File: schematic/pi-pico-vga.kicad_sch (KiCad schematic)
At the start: 33 parts, among them J1 VGA, J2 USB Keyboard, J3 Micro_SD_Card, J4 Power, J5 UART, J6 External, J7 Jack-DC, SW1 Power switch, SW2 User, SW3 Microswitch, U1 DS1307+, U2 Level Shift, Y1 32.768 Hz

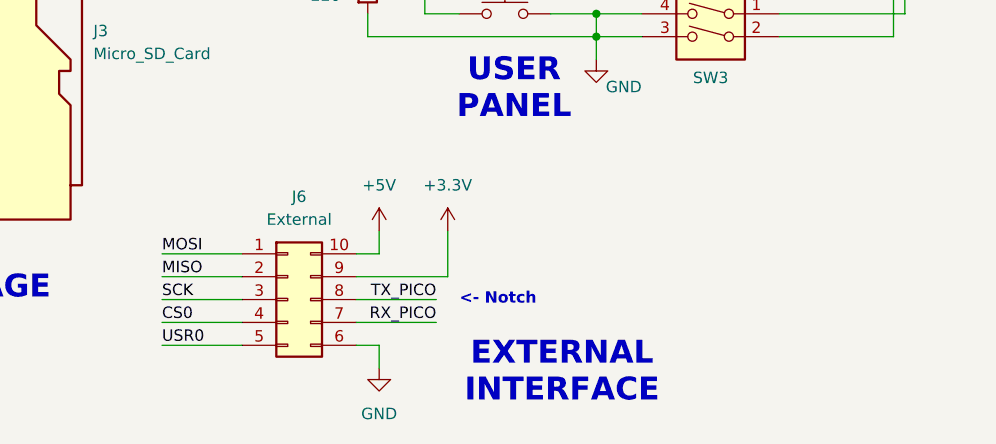
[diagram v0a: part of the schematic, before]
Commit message: .
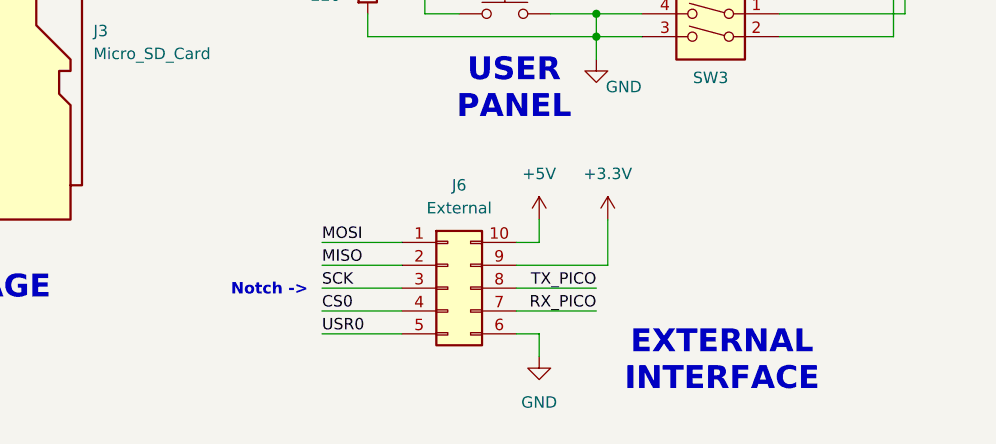
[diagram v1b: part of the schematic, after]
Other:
- note added: "Notch ->"
- note removed: "<- Notch"
- moved on the sheet: J6
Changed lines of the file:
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@@
 	(text "EXTERNAL\nINTERFACE"
 		(exclude_from_sim no)
-		(at 115.57 191.008 0)
+		(at 133.35 189.738 0)
 		(effects
 			(font
@@
 		)
 	)
-	(text "<- Notch"
+	(text "USER\nPANEL"
 		(exclude_from_sim no)
-		(at 108.458 182.88 0)
+		(at 110.236 159.512 0)
 		(effects
 			(font
-				(size 1.27 1.27)
-				(thickness 0.254)
+				(size 2.54 2.54)
+				(thickness 0.508)
 				(bold yes)
 			)
 		)
 	)
-	(text "USER\nPANEL"
+	(text "Notch ->"
 		(exclude_from_sim no)
-		(at 110.236 159.512 0)
+		(at 83.058 181.864 0)
 		(effects
 			(font
-				(size 2.54 2.54)
-				(thickness 0.508)
+				(size 1.27 1.27)
+				(thickness 0.254)
 				(bold yes)
 			)
@@
 	(wire
 		(pts
-			(xy 102.87 175.26) (xy 102.87 180.34)
+			(xy 120.65 173.99) (xy 120.65 179.07)
 		)
 		(stroke
@@
 	(wire
 		(pts
-			(xy 102.87 180.34) (xy 92.71 180.34)
+			(xy 120.65 179.07) (xy 110.49 179.07)
 		)
 		(stroke
@@
 	(wire
 		(pts
-			(xy 95.25 177.8) (xy 92.71 177.8)
+			(xy 113.03 176.53) (xy 110.49 176.53)
 		)
 		(stroke
@@
 	(wire
 		(pts
-			(xy 71.12 180.34) (xy 80.01 180.34)
+			(xy 88.9 179.07) (xy 97.79 179.07)
 		)
 		(stroke
@@
 	(wire
 		(pts
-			(xy 71.12 177.8) (xy 80.01 177.8)
+			(xy 88.9 176.53) (xy 97.79 176.53)
 		)
 		(stroke
@@
 	(wire
 		(pts
-			(xy 95.25 190.5) (xy 95.25 187.96)
+			(xy 113.03 189.23) (xy 113.03 186.69)
 		)
 		(stroke
@@
 	(wire
 		(pts
-			(xy 71.12 182.88) (xy 80.01 182.88)
+			(xy 88.9 181.61) (xy 97.79 181.61)
 		)
 		(stroke
@@
 	(wire
 		(pts
-			(xy 95.25 175.26) (xy 95.25 177.8)
+			(xy 113.03 173.99) (xy 113.03 176.53)
 		)
 		(stroke
@@
 	(wire
 		(pts
-			(xy 95.25 187.96) (xy 92.71 187.96)
+			(xy 113.03 186.69) (xy 110.49 186.69)
 		)
 		(stroke
@@
 	(wire
 		(pts
-			(xy 101.6 182.88) (xy 92.71 182.88)
+			(xy 119.38 181.61) (xy 110.49 181.61)
 		)
 		(stroke
@@
 	(wire
 		(pts
-			(xy 71.12 187.96) (xy 80.01 187.96)
+			(xy 88.9 186.69) (xy 97.79 186.69)
 		)
 		(stroke
@@
 	(wire
 		(pts
-			(xy 71.12 185.42) (xy 80.01 185.42)
+			(xy 88.9 184.15) (xy 97.79 184.15)
 		)
 		(stroke
@@
 	(wire
 		(pts
-			(xy 101.6 185.42) (xy 92.71 185.42)
+			(xy 119.38 184.15) (xy 110.49 184.15)
 		)
 		(stroke
@@
 	)
 	(label "RX_PICO"
-		(at 101.6 185.42 180)
+		(at 119.38 184.15 180)
 		(effects
 			(font
@@
 	)
 	(label "MISO"
-		(at 71.12 180.34 0)
+		(at 88.9 179.07 0)
 		(effects
 			(font
@@
 	)
 	(label "USR0"
-		(at 71.12 187.96 0)
+		(at 88.9 186.69 0)
 		(effects
 			(font
@@
 	)
 	(label "SCK"
-		(at 71.12 182.88 0)
+		(at 88.9 181.61 0)
 		(effects
 			(font
@@
 	)
 	(label "TX_PICO"
-		(at 101.6 182.88 180)
+		(at 119.38 181.61 180)
 		(effects
 			(font
@@
 	)
 	(label "CS0"
-		(at 71.12 185.42 0)
+		(at 88.9 184.15 0)
 		(effects
 			(font
@@
 	)
 	(label "MOSI"
-		(at 71.12 177.8 0)
+		(at 88.9 176.53 0)
 		(effects
 			(font
@@
 	(symbol
 		(lib_id "power:+3.3V")
-		(at 102.87 175.26 0)
+		(at 120.65 173.99 0)
 		(unit 1)
 		(exclude_from_sim no)
@@
 		(fields_autoplaced yes)
 		(property "Reference" "#PWR021"
-			(at 102.87 179.07 0)
+			(at 120.65 177.8 0)
 			(effects
 				(font
@@
 		)
 		(property "Value" "+3.3V"
-			(at 102.87 170.18 0)
+			(at 120.65 168.91 0)
 			(effects
 				(font
@@
 		)
 		(property "Footprint" ""
-			(at 102.87 175.26 0)
+			(at 120.65 173.99 0)
 			(effects
 				(font
@@
 		)
 		(property "Datasheet" ""
-			(at 102.87 175.26 0)
+			(at 120.65 173.99 0)
 			(effects
 				(font
@@
 		)
 		(property "Description" "Power symbol creates a global label with name \"+3.3V\""
-			(at 102.87 175.26 0)
+			(at 120.65 173.99 0)
 			(effects
 				(font
@@
 	(symbol
 		(lib_id "power:GND")
-		(at 95.25 190.5 0)
+		(at 113.03 189.23 0)
 		(unit 1)
 		(exclude_from_sim no)
@@
 		(fields_autoplaced yes)
 		(property "Reference" "#PWR017"
-			(at 95.25 196.85 0)
+			(at 113.03 195.58 0)
 			(effects
 				(font
@@
 		)
 		(property "Value" "GND"
-			(at 95.25 195.58 0)
+			(at 113.03 194.31 0)
 			(effects
 				(font
@@
 		)
 		(property "Footprint" ""
-			(at 95.25 190.5 0)
+			(at 113.03 189.23 0)
 			(effects
 				(font
@@
 		)
 		(property "Datasheet" ""
-			(at 95.25 190.5 0)
+			(at 113.03 189.23 0)
 			(effects
 				(font
@@
 		)
 		(property "Description" "Power symbol creates a global label with name \"GND\" , ground"
-			(at 95.25 190.5 0)
+			(at 113.03 189.23 0)
 			(effects
 				(font
@@
 	(symbol
 		(lib_id "power:+5V")
-		(at 95.25 175.26 0)
+		(at 113.03 173.99 0)
 		(unit 1)
 		(exclude_from_sim no)
@@
 		(fields_autoplaced yes)
 		(property "Reference" "#PWR020"
-			(at 95.25 179.07 0)
+			(at 113.03 177.8 0)
 			(effects
 				(font
@@
 		)
 		(property "Value" "+5V"
-			(at 95.25 170.18 0)
+			(at 113.03 168.91 0)
 			(effects
 				(font
@@
 		)
 		(property "Footprint" ""
-			(at 95.25 175.26 0)
+			(at 113.03 173.99 0)
 			(effects
 				(font
@@
 		)
 		(property "Datasheet" ""
-			(at 95.25 175.26 0)
+			(at 113.03 173.99 0)
 			(effects
 				(font
@@
 		)
 		(property "Description" "Power symbol creates a global label with name \"+5V\""
-			(at 95.25 175.26 0)
+			(at 113.03 173.99 0)
 			(effects
 				(font
@@
 	(symbol
 		(lib_id "Connector_Generic:Conn_02x05_Counter_Clockwise")
-		(at 85.09 182.88 0)
+		(at 102.87 181.61 0)
 		(unit 1)
 		(exclude_from_sim no)
@@
 		(fields_autoplaced yes)
 		(property "Reference" "J6"
-			(at 86.36 171.45 0)
+			(at 104.14 170.18 0)
 			(effects
 				(font
@@
 		)
 		(property "Value" "External"
-			(at 86.36 173.99 0)
+			(at 104.14 172.72 0)
 			(effects
 				(font
@@
 		)
 		(property "Footprint" ""
-			(at 85.09 182.88 0)
+			(at 102.87 181.61 0)
 			(effects
 				(font
@@
 		)
 		(property "Datasheet" "~"
-			(at 85.09 182.88 0)
+			(at 102.87 181.61 0)
 			(effects
 				(font
@@
 		)
 		(property "Description" "Generic connector, double row, 02x05, counter clockwise pin numbering scheme (similar to DIP package numbering), script generated (kicad-library-utils/schlib/autogen/connector/)"
-			(at 85.09 182.88 0)
+			(at 102.87 181.61 0)
 			(effects
 				(font

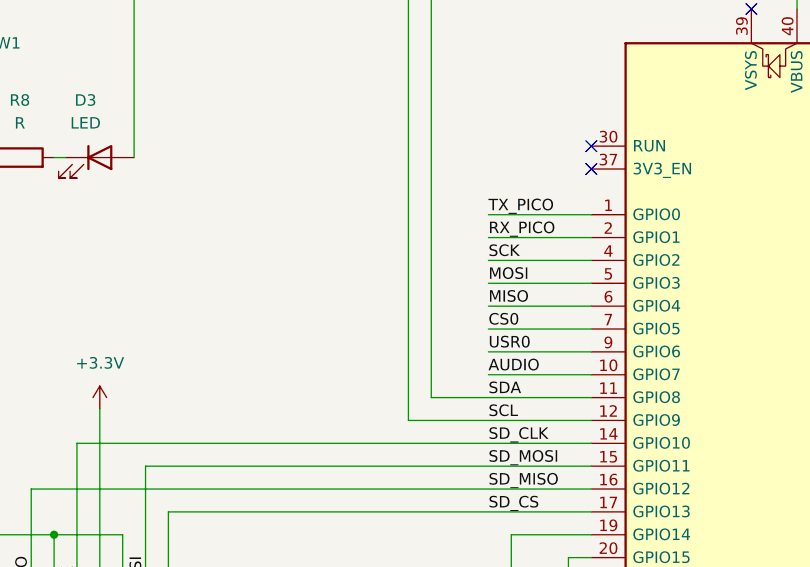
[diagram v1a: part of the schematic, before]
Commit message: .
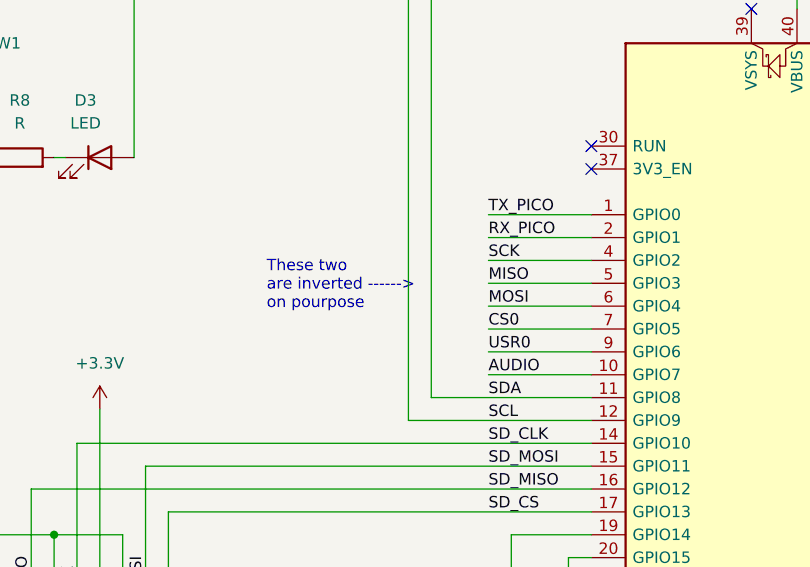
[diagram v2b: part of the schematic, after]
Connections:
- net MISO: now also A1.5 (GPIO3); no longer A1.6 (GPIO4)
- net MOSI: now also A1.6 (GPIO4); no longer A1.5 (GPIO3)
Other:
- note added: "These two are inverted ------> on pourpose"
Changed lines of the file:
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@@
+		)
+	)
+	(text "These two\nare inverted ------>\non pourpose"
+		(exclude_from_sim no)
+		(at 66.802 91.694 0)
+		(effects
+			(font
+				(size 1.27 1.27)
+			)
+			(justify left)
 		)
 	)
@@
 		)
 	)
-	(label "MISO"
+	(label "MOSI"
 		(at 91.44 93.98 0)
 		(effects
@@
 		)
 	)
-	(label "MOSI"
+	(label "MISO"
 		(at 91.44 91.44 0)
 		(effects
